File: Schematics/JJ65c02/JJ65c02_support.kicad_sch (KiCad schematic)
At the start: 37 parts, among them J1 AudioJack, U10 VIA Port Shifter, U11 Misc Shifter, U5 TLV2217-33KCSE3, U9 Data Level Shifter, X1 1Mhz, X2 1.8Mhz

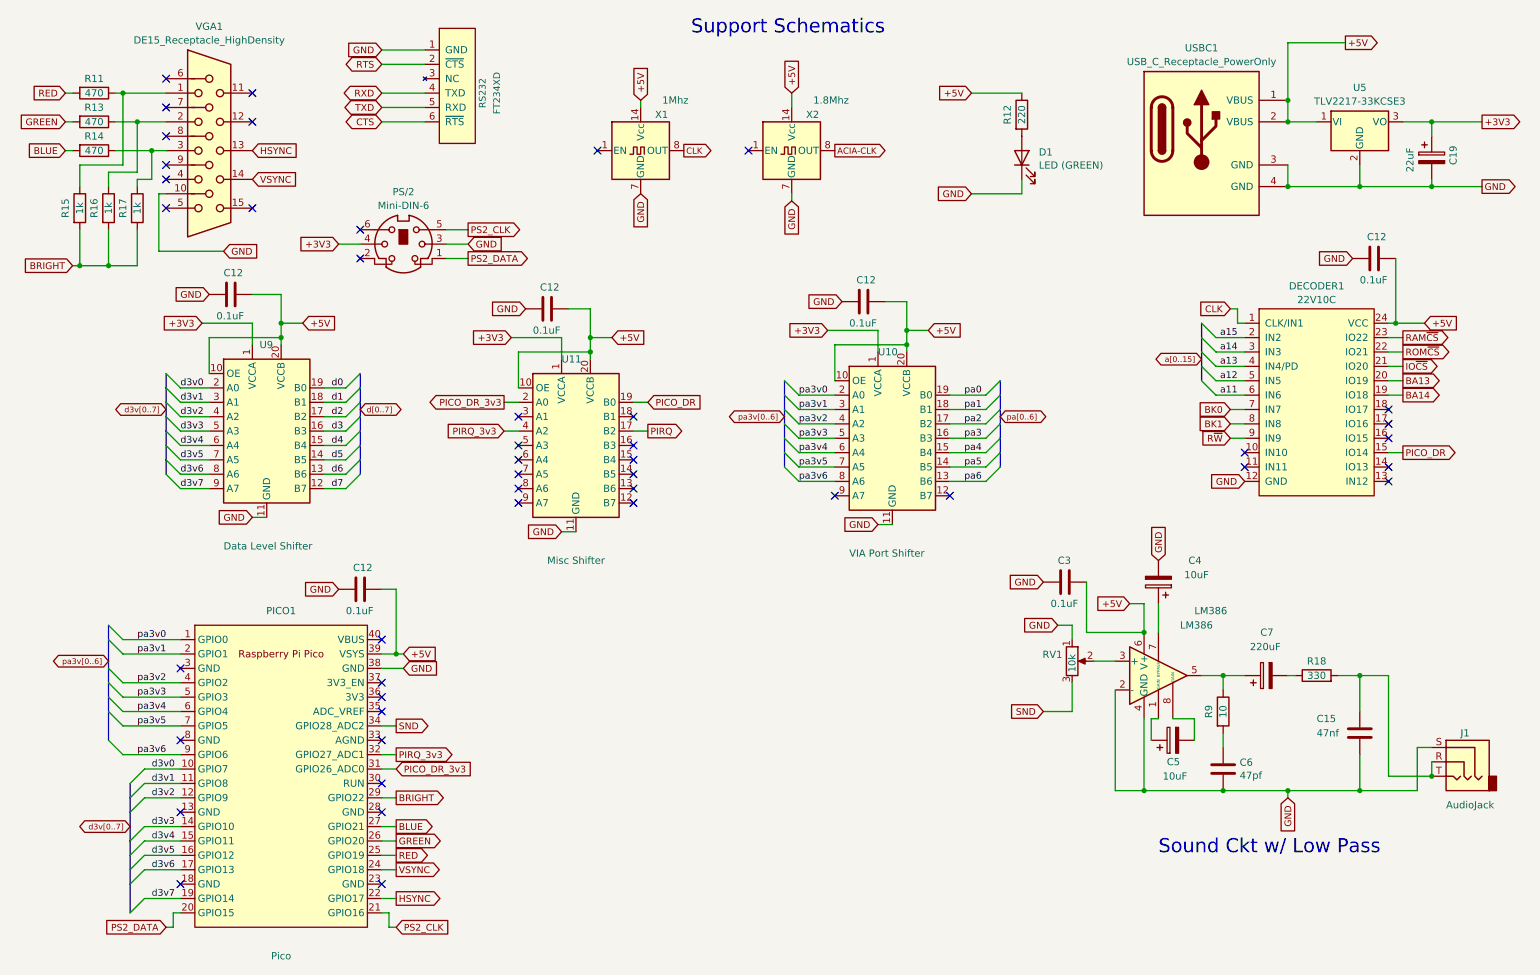
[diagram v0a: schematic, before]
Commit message: Update demo
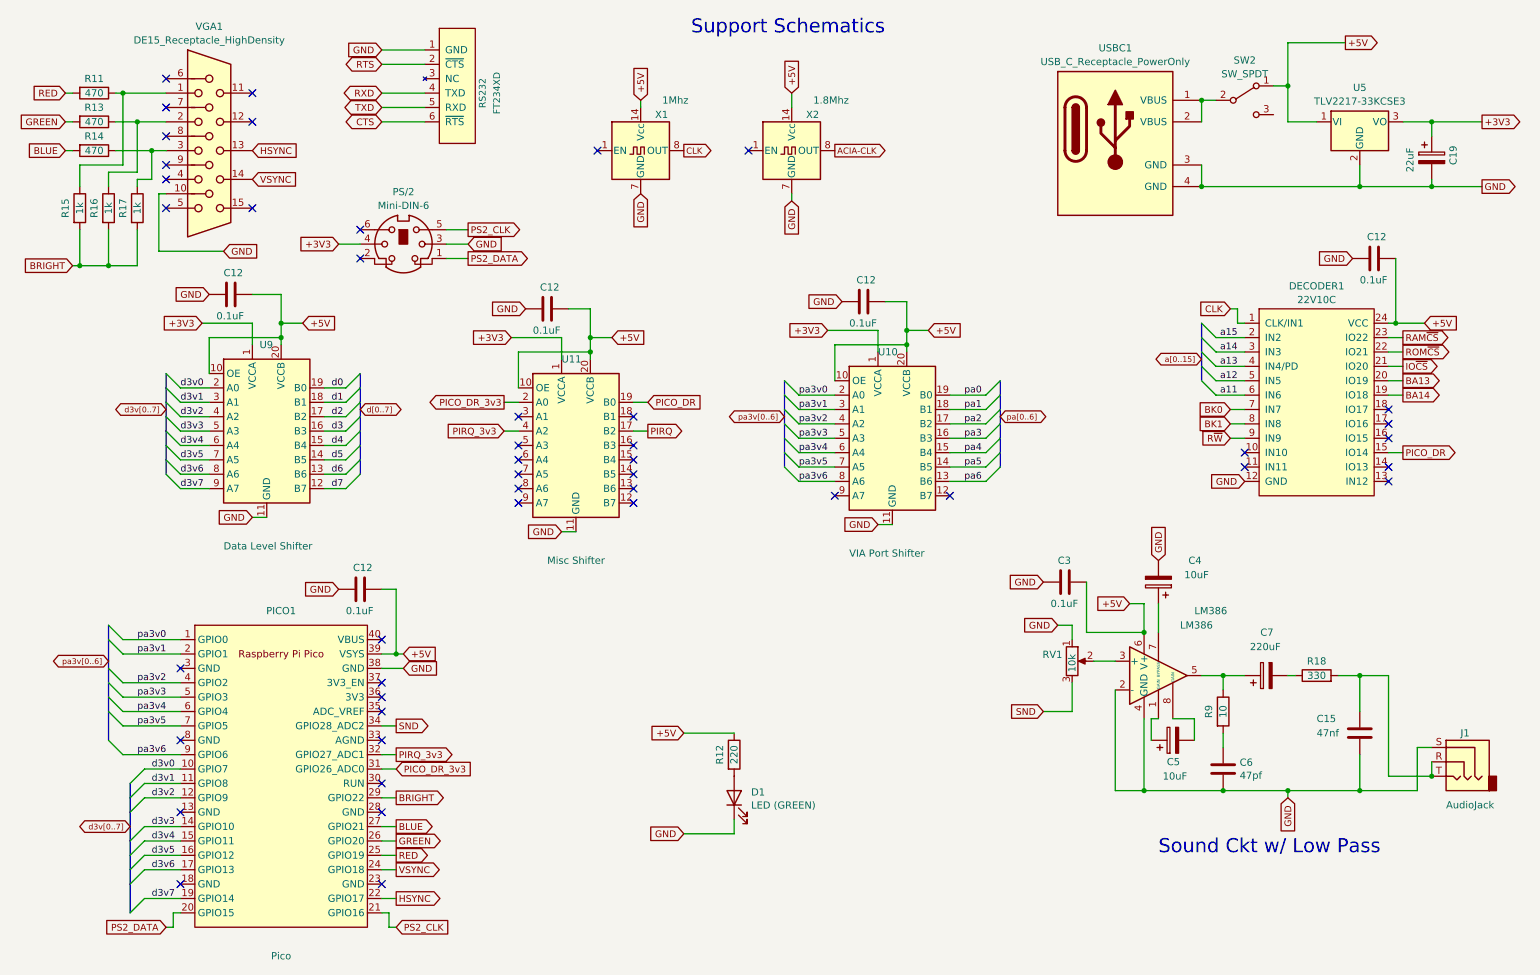
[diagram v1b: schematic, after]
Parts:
- added SW2: SW_SPDT, symbol Switch:SW_SPDT
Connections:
- net +5V: now also SW2.1 (A); no longer USBC1.1 (VBUS), USBC1.2 (VBUS)
- new net: SW2.2 (B), USBC1.1 (VBUS), USBC1.2 (VBUS)
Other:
- moved on the sheet: D1, R12, USBC1
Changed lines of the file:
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@@
   (junction (at 262.89 33.02) (diameter 0) (color 0 0 0 0)
   )
-  (junction (at 237.49 44.45) (diameter 0) (color 0 0 0 0)
+  (junction (at 222.25 29.21) (diameter 0) (color 0 0 0 0)
   )
   (junction (at 212.09 123.19) (diameter 0) (color 0 0 0 0)
@@
   (junction (at 114.3 71.12) (diameter 0) (color 0 0 0 0)
   )
-  (junction (at 237.49 33.02) (diameter 0) (color 0 0 0 0)
-  )
   (junction (at 170.18 72.39) (diameter 0) (color 0 0 0 0)
   )
@@
   (junction (at 262.89 44.45) (diameter 0) (color 0 0 0 0)
   )
-  (junction (at 237.49 29.21) (diameter 0) (color 0 0 0 0)
-  )
   (junction (at 250.19 130.81) (diameter 0) (color 0 0 0 0)
   )
@@
   )
   (junction (at 114.3 73.66) (diameter 0) (color 0 0 0 0)
+  )
+  (junction (at 237.49 26.67) (diameter 0) (color 0 0 0 0)
+  )
+  (junction (at 222.25 44.45) (diameter 0) (color 0 0 0 0)
   )
   (junction (at 256.54 68.58) (diameter 0) (color 0 0 0 0)
@@
     (stroke (width 0) (type default))
   )
+  (wire (pts (xy 222.25 29.21) (xy 222.25 33.02))
+    (stroke (width 0) (type default))
+  )
   (bus (pts (xy 148.59 88.9) (xy 148.59 91.44))
     (stroke (width 0) (type default))
@@
     (stroke (width 0) (type default))
   )
+  (wire (pts (xy 237.49 26.67) (xy 237.49 33.02))
+    (stroke (width 0) (type default))
+  )
   (bus (pts (xy 73.66 77.47) (xy 73.66 80.01))
     (stroke (width 0) (type default))
@@
     (stroke (width 0) (type default))
   )
-  (wire (pts (xy 181.61 45.72) (xy 190.5 45.72))
+  (wire (pts (xy 130.81 158.75) (xy 139.7 158.75))
     (stroke (width 0) (type default))
   )
@@
     (stroke (width 0) (type default))
   )
-  (wire (pts (xy 237.49 44.45) (xy 250.19 44.45))
+  (wire (pts (xy 222.25 44.45) (xy 250.19 44.45))
     (stroke (width 0) (type default))
   )
@@
     (stroke (width 0) (type default))
   )
+  (wire (pts (xy 234.95 26.67) (xy 237.49 26.67))
+    (stroke (width 0) (type default))
+  )
   (wire (pts (xy 151.13 86.36) (xy 157.48 86.36))
     (stroke (width 0) (type default))
@@
     (stroke (width 0) (type default))
   )
-  (wire (pts (xy 181.61 27.94) (xy 190.5 27.94))
+  (wire (pts (xy 130.81 140.97) (xy 139.7 140.97))
     (stroke (width 0) (type default))
   )
@@
     (stroke (width 0) (type default))
   )
+  (wire (pts (xy 222.25 40.64) (xy 222.25 44.45))
+    (stroke (width 0) (type default))
+  )
   (wire (pts (xy 40.64 172.72) (xy 40.64 175.26))
     (stroke (width 0) (type default))
@@
     (stroke (width 0) (type default))
   )
-  (wire (pts (xy 190.5 45.72) (xy 190.5 43.18))
+  (wire (pts (xy 222.25 29.21) (xy 224.79 29.21))
+    (stroke (width 0) (type default))
+  )
+  (wire (pts (xy 139.7 158.75) (xy 139.7 156.21))
     (stroke (width 0) (type default))
   )
@@
     (stroke (width 0) (type default))
   )
-  (wire (pts (xy 237.49 40.64) (xy 237.49 44.45))
-    (stroke (width 0) (type default))
-  )
   (bus (pts (xy 73.66 85.09) (xy 73.66 87.63))
     (stroke (width 0) (type default))
@@
     (stroke (width 0) (type default))
   )
-  (wire (pts (xy 237.49 29.21) (xy 237.49 33.02))
+  (wire (pts (xy 237.49 19.05) (xy 237.49 26.67))
     (stroke (width 0) (type default))
   )
@@
   )
   (bus (pts (xy 73.66 90.17) (xy 73.66 92.71))
-    (stroke (width 0) (type default))
-  )
-  (wire (pts (xy 237.49 19.05) (xy 237.49 29.21))
     (stroke (width 0) (type default))
   )
@@
     )
   )
-  (global_label "+5V" (shape input) (at 181.61 27.94 180) (fields_autoplaced)
-    (effects (font (size 1.1938 1.1938)) (justify right))
-    (property "Intersheetrefs" "${INTERSHEET_REFS}" (at 123.19 -50.8 0)
+  (global_label "+5V" (shape input) (at 130.81 140.97 180) (fields_autoplaced)
+    (effects (font (size 1.1938 1.1938)) (justify right))
+    (property "Intersheetrefs" "${INTERSHEET_REFS}" (at 72.39 62.23 0)
       (effects (font (size 1.27 1.27)) hide)
     )
@@
     )
   )
-  (global_label "GND" (shape input) (at 181.61 45.72 180) (fields_autoplaced)
-    (effects (font (size 1.1938 1.1938)) (justify right))
-    (property "Intersheetrefs" "${INTERSHEET_REFS}" (at 123.19 -50.8 0)
+  (global_label "GND" (shape input) (at 130.81 158.75 180) (fields_autoplaced)
+    (effects (font (size 1.1938 1.1938)) (justify right))
+    (property "Intersheetrefs" "${INTERSHEET_REFS}" (at 72.39 62.23 0)
       (effects (font (size 1.27 1.27)) hide)
     )
@@
     )
   )
-  (symbol (lib_id "Device:LED") (at 190.5 39.37 90) (unit 1)
-    (in_bom yes) (on_board yes) (dnp no)
-    (property "Reference" "D1" (at 193.4972 38.3794 90)
+  (symbol (lib_id "Device:LED") (at 139.7 152.4 90) (unit 1)
+    (in_bom yes) (on_board yes) (dnp no)
+    (property "Reference" "D1" (at 142.6972 151.4094 90)
       (effects (font (size 1.27 1.27)) (justify right))
     )
-    (property "Value" "LED (GREEN)" (at 193.4972 40.6908 90)
+    (property "Value" "LED (GREEN)" (at 142.6972 153.7208 90)
       (effects (font (size 1.27 1.27)) (justify right))
     )
-    (property "Footprint" "LED_THT:LED_D3.0mm_FlatTop" (at 190.5 39.37 0)
-      (effects (font (size 1.27 1.27)) hide)
-    )
-    (property "Datasheet" "~" (at 190.5 39.37 0)
+    (property "Footprint" "LED_THT:LED_D3.0mm_FlatTop" (at 139.7 152.4 0)
+      (effects (font (size 1.27 1.27)) hide)
+    )
+    (property "Datasheet" "~" (at 139.7 152.4 0)
       (effects (font (size 1.27 1.27)) hide)
     )
@@
     )
   )
-  (symbol (lib_id "Device:R") (at 190.5 31.75 0) (unit 1)
-    (in_bom yes) (on_board yes) (dnp no)
-    (property "Reference" "R12" (at 187.96 31.75 90)
-      (effects (font (size 1.27 1.27)))
-    )
-    (property "Value" "220" (at 190.5 31.75 90)
-      (effects (font (size 1.27 1.27)))
-    )
-    (property "Footprint" "Resistor_THT:R_Axial_DIN0207_L6.3mm_D2.5mm_P7.62mm_Horizontal" (at 188.722 31.75 90)
-      (effects (font (size 1.27 1.27)) hide)
-    )
-    (property "Datasheet" "~" (at 190.5 31.75 0)
+  (symbol (lib_id "Device:R") (at 139.7 144.78 0) (unit 1)
+    (in_bom yes) (on_board yes) (dnp no)
+    (property "Reference" "R12" (at 137.16 144.78 90)
+      (effects (font (size 1.27 1.27)))
+    )
+    (property "Value" "220" (at 139.7 144.78 90)
+      (effects (font (size 1.27 1.27)))
+    )
+    (property "Footprint" "Resistor_THT:R_Axial_DIN0207_L6.3mm_D2.5mm_P7.62mm_Horizontal" (at 137.922 144.78 90)
+      (effects (font (size 1.27 1.27)) hide)
+    )
+    (property "Datasheet" "~" (at 139.7 144.78 0)
       (effects (font (size 1.27 1.27)) hide)
     )
@@
         (path "/2db910a0-b943-40b4-b81f-068ba5265f56/00000000-0000-0000-0000-000061660cac"
           (reference "R15") (unit 1)
+        )
+      )
+    )
+  )
+  (symbol (lib_id "Switch:SW_SPDT") (at 229.87 29.21 0) (unit 1)
+    (in_bom yes) (on_board yes) (dnp no) (fields_autoplaced)
+    (property "Reference" "SW2" (at 229.87 22.1447 0)
+      (effects (font (size 1.27 1.27)))
+    )
+    (property "Value" "SW_SPDT" (at 229.87 24.5689 0)
+      (effects (font (size 1.27 1.27)))
+    )
+    (property "Footprint" "" (at 229.87 29.21 0)
+      (effects (font (size 1.27 1.27)) hide)
+    )
+    (property "Datasheet" "~" (at 229.87 29.21 0)
+      (effects (font (size 1.27 1.27)) hide)
+    )
+    (pin "1")
+    (pin "2")
+    (pin "3")
+    (instances
+      (project "JJ65c02"
+        (path "/2db910a0-b943-40b4-b81f-068ba5265f56/00000000-0000-0000-0000-000061660cac"
+          (reference "SW2") (unit 1)
         )
       )
@@
     )
   )
-  (symbol (lib_id "Connector:USB_C_Receptacle_PowerOnly_6P") (at 222.25 36.83 0) (unit 1)
+  (symbol (lib_id "Connector:USB_C_Receptacle_PowerOnly_6P") (at 207.01 36.83 0) (unit 1)
     (in_bom yes) (on_board yes) (dnp no) (fields_autoplaced)
-    (property "Reference" "USBC1" (at 222.25 19.9857 0)
-      (effects (font (size 1.27 1.27)))
-    )
-    (property "Value" "USB_C_Receptacle_PowerOnly" (at 222.25 22.4099 0)
-      (effects (font (size 1.27 1.27)))
-    )
-    (property "Footprint" "JJ65c02:USBC_power" (at 226.06 34.29 0)
-      (effects (font (size 1.27 1.27)) hide)
-    )
-    (property "Datasheet" "https://www.usb.org/sites/default/files/documents/usb_type-c.zip" (at 223.52 50.8 0)
-      (effects (font (size 1.27 1.27)) hide)
-    )
+    (property "Reference" "USBC1" (at 207.01 19.9857 0)
+      (effects (font (size 1.27 1.27)))
+    )
+    (property "Value" "USB_C_Receptacle_PowerOnly" (at 207.01 22.4099 0)
+      (effects (font (size 1.27 1.27)))
+    )
+    (property "Footprint" "JJ65c02:USBC_power" (at 210.82 34.29 0)
+      (effects (font (size 1.27 1.27)) hide)
+    )
+    (property "Datasheet" "https://www.usb.org/sites/default/files/documents/usb_type-c.zip" (at 208.28 50.8 0)
+      (effects (font (size 1.27 1.27)) hide)
+    )
